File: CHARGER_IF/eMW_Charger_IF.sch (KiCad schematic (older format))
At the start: 9 parts

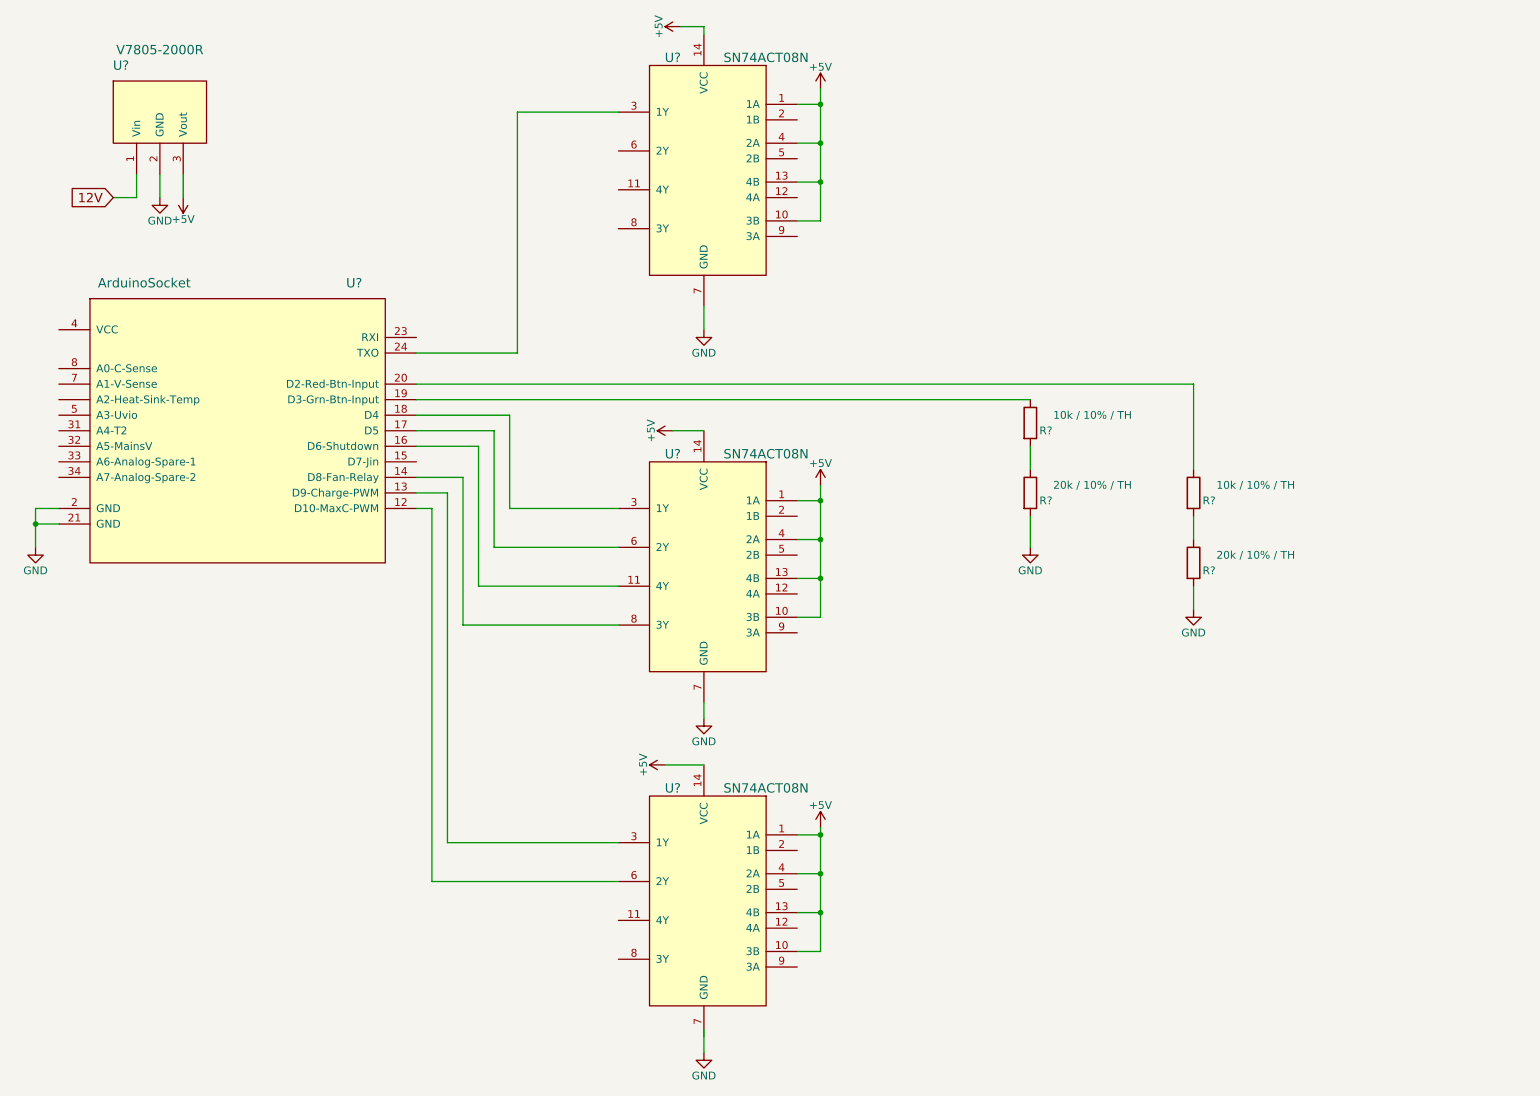
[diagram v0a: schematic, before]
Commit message: Charger IF WIP
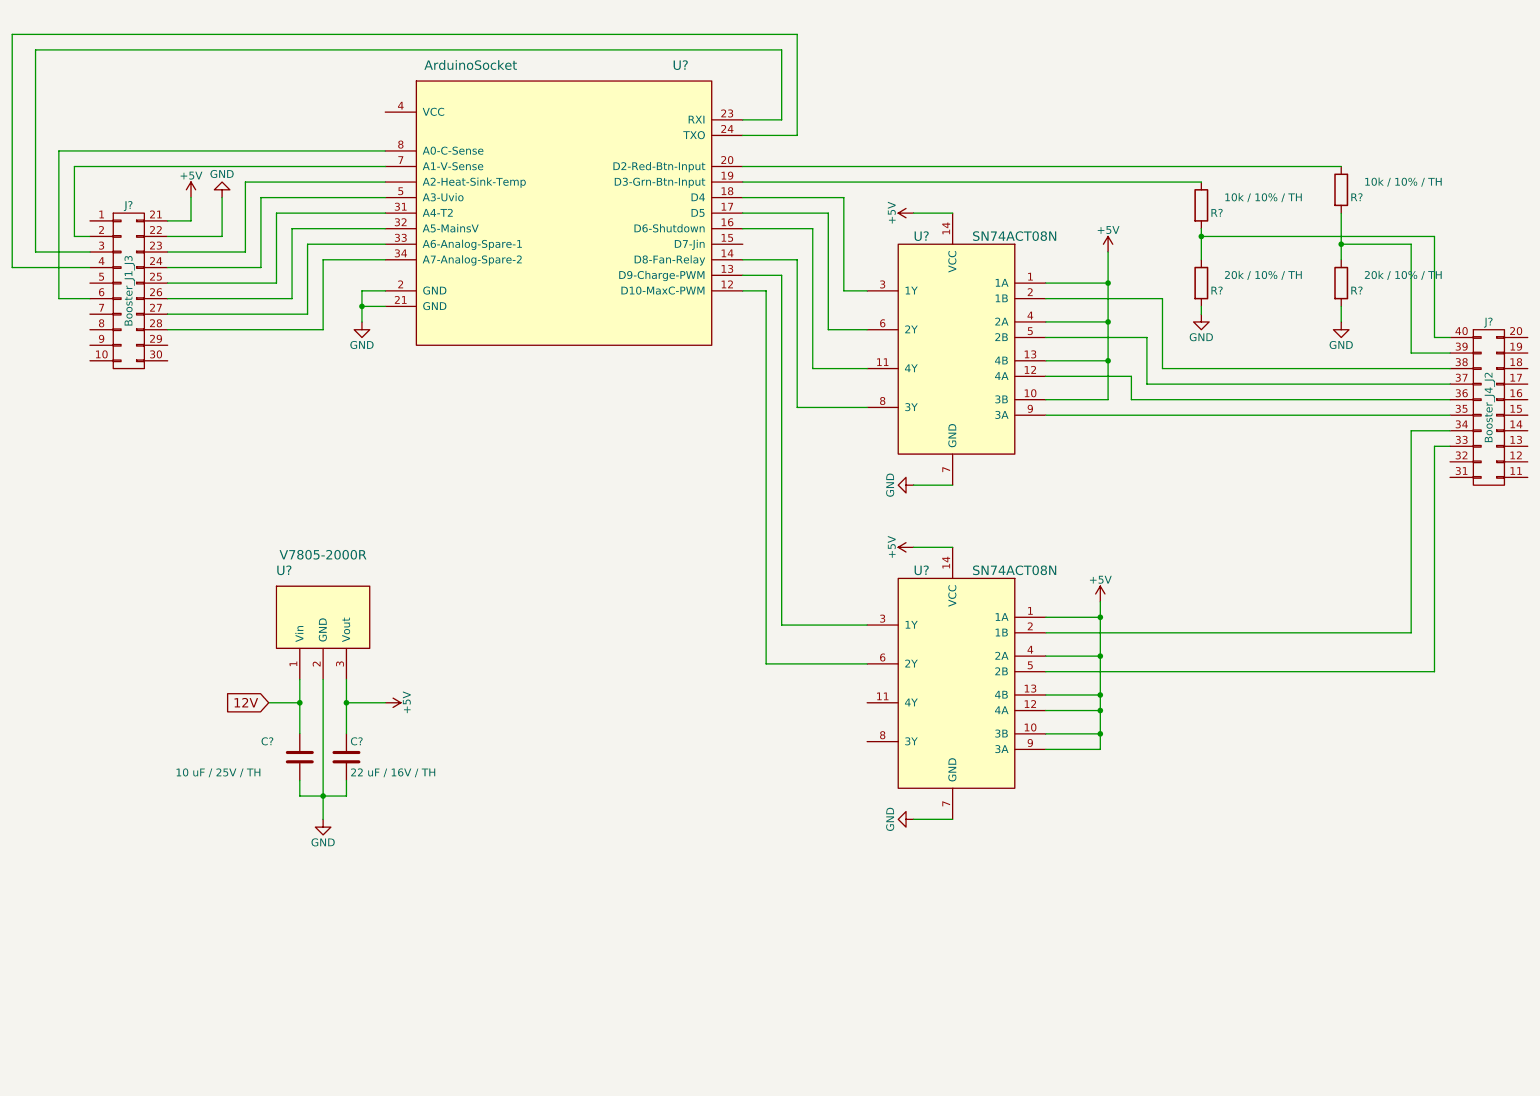
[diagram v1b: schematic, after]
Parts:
- removed U?: SN74ACT08N, symbol SN74LS08N
- added C?: 10 uF / 25V / TH, symbol C
- added C?: 22 uF / 16V / TH, symbol C
- added J?: Booster_J1_J3, symbol Booster_J1_J3
- added J?: Booster_J4_J2, symbol Booster_J4_J2
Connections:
- net +5V: now also U?.12 (4A), U?.9 (3A), C?.1, J?.21 (P21)
- net 12V: now also C?.1
- net GND: now also U?.7 (GND), C?.2, C?.2, J?.22 (P22)
- net at U?.23 (RXI): now also J?.3 (P3)
- net at U?.24 (TXO): now also J?.4 (P4)
- net at U?.31 (A4-T2): now also J?.25 (P25)
- net at U?.32 (A5-MainsV): now also J?.26 (P26)
- net at U?.33 (A6-Analog-Spare-1): now also J?.27 (P27)
- net at U?.34 (A7-Analog-Spare-2): now also J?.28 (P28)
- net at U?.5 (A3-Uvio): now also J?.24 (P24)
- net at U?.7 (A1-V-Sense): now also J?.2 (P2)
- net at U?.8 (A0-C-Sense): now also J?.6 (P6)
- net at U?.~ (A2-Heat-Sink-Temp): now also J?.23 (P23)
- net at U?.12 (4A): now also J?.36 (P36)
- net at U?.2 (1B): now also J?.38 (P38)
- net at U?.5 (2B): now also J?.37 (P37)
- net at U?.9 (3A): now also J?.35 (P35)
- net at U?.2 (1B): now also J?.34 (P34)
- net at U?.5 (2B): now also J?.33 (P33)
- net at R?.1, R?.2: now also J?.39 (P39)
- net at R?.1, R?.2: now also J?.40 (P40)
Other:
- moved on the sheet: R?, U?
